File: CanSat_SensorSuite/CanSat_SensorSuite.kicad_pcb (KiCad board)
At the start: 4 copper layers, 100 x 80 mm, 42 parts, among them J13 Conn_02x03_Odd_Even, J2 USBC_Conn, J4 Pin_01x02, U1 RP2350_80QFN, U2 S25FL128, U3 NCP1117_3.3, X1 ABM8-272-T3

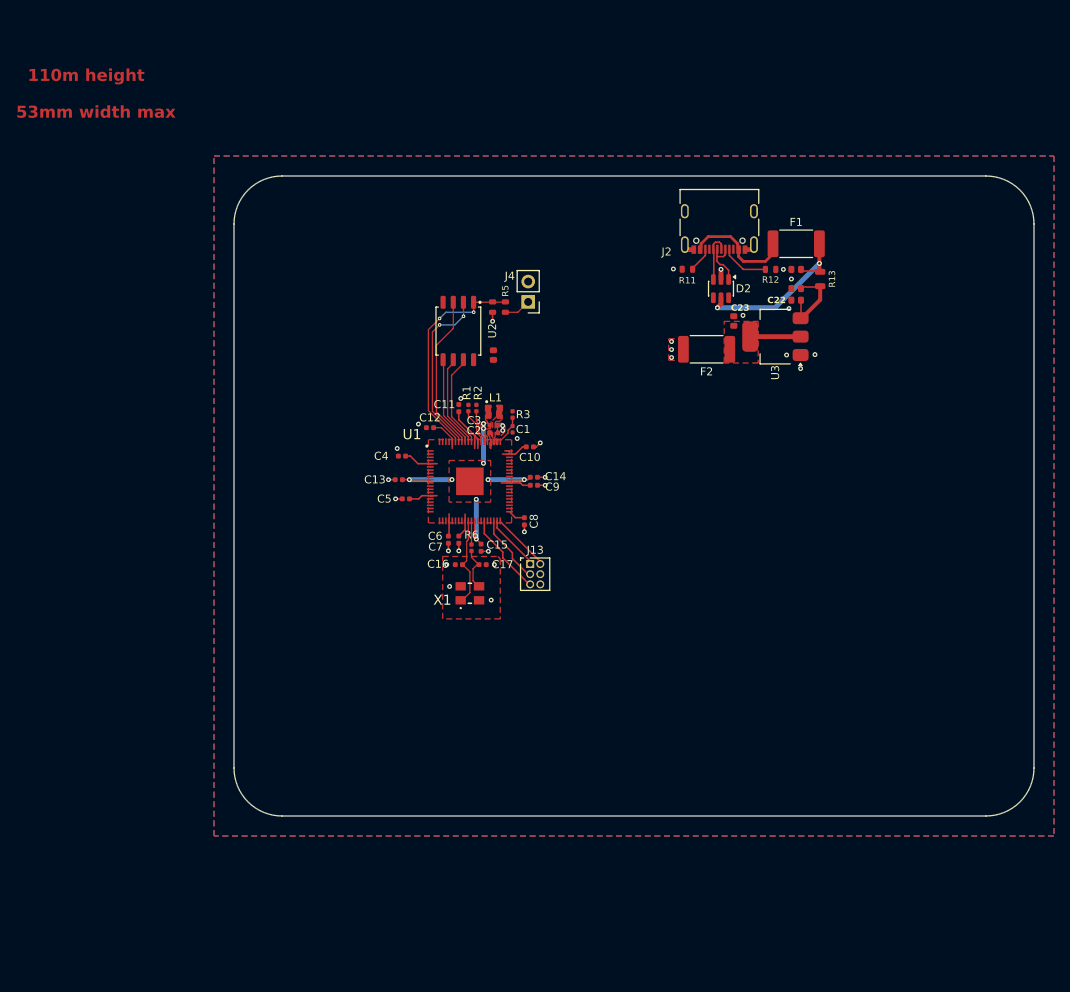
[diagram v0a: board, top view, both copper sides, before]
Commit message: Major sensor suite board changes, start of PCB layout
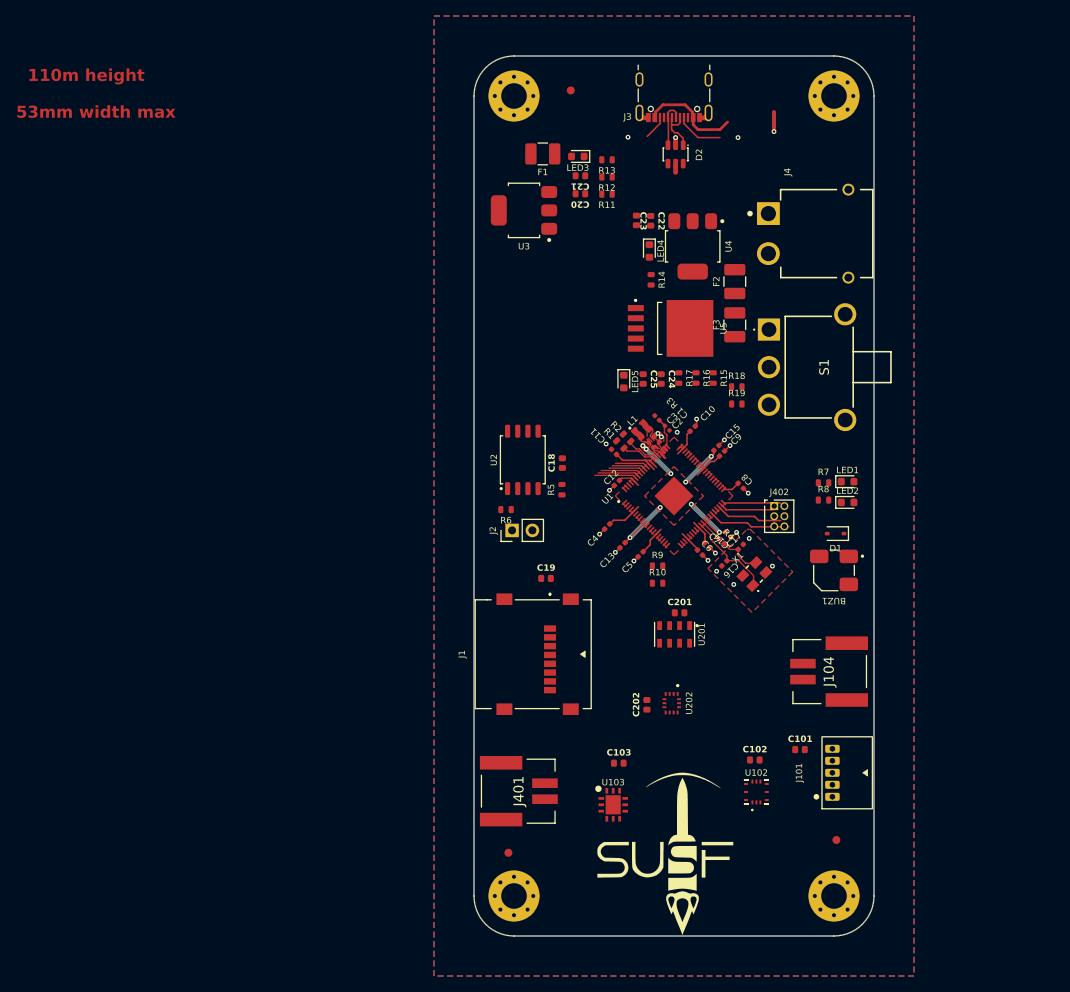
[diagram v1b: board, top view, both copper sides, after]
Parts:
- removed J13: Conn_02x03_Odd_Even, 0_Connectors:PinHeader_2x03_P1.27mm_Vertical
- added BUZ1: ~, 0_Passives:BUZZER,5x5mm, F.Cu at (175.0, 99.3)
- added C101: 100nF, 0_Capacitors:C_0603_1608_DensityHigh, F.Cu at (170.8, 121.7)
- added C102: 100nF, 0_Capacitors:C_0603_1608_DensityHigh, F.Cu at (165.1, 123.0)
- added C103: 100nF, 0_Capacitors:C_0603_1608_DensityHigh, F.Cu at (148.1, 123.4)
- added C19: 100nF, 0_Capacitors:C_0603_1608_DensityHigh, F.Cu at (139.0, 100.3)
- added C201: 100nF, 0_Capacitors:C_0603_1608_DensityHigh, F.Cu at (155.7, 104.6)
- added C202: 100nF, 0_Capacitors:C_0603_1608_DensityHigh, F.Cu at (151.6, 116.1)
- added C24: 10uF, 0_Capacitors:C_0603_1608_DensityHigh, F.Cu at (153.4, 75.4)
- added C25: 10uF, 0_Capacitors:C_0603_1608_DensityHigh, F.Cu at (151.2, 75.4)
- added D1: ~, 0_Passives:D_SOD-323, F.Cu at (175.2, 94.7)
- added F3: Fuse, 0_Power:Fuse_1210_3225Metric, F.Cu at (162.6, 68.6)
- added FID301: Fiducial Marker, 0_Mechanical:Fiducial_1mm_Mask2mm, F.Cu at (134.3, 134.6)
- added FID302: Fiducial Marker, 0_Mechanical:Fiducial_1mm_Mask2mm, F.Cu at (175.3, 133.0)
- added FID303: Fiducial Marker, 0_Mechanical:Fiducial_1mm_Mask2mm, F.Cu at (142.1, 39.3)
- added G***: LOGO, SUSF_Footprint_Lib:SUSF_LOGO_BIG, F.Cu at (154.4, 134.8)
- added J1: Micro_SD_Card, 0_Connectors:Molex_472192001_uSD, F.Cu at (137.7, 109.8)
- added J101: SPS30, 0_Connectors:JST-S5B-ZR, F.Cu at (174.8, 127.6)
- added J104: Molex_01x02, 0_Connectors:502352_0201, F.Cu at (173.9, 112.0)
- added J3: USBC_Conn, 0_Connectors:USB4105_GCT, F.Cu at (155.0, 39.3)
- added J401: Molex_01x02, 0_Connectors:502352_0201, F.Cu at (136.1, 126.9)
- added J402: Conn_02x03, 0_Connectors:PinHeader_2x03_P1.27mm_Vertical, F.Cu at (167.5, 91.3)
- added LED1: Green, 0_Passives:LED_0603_1608Metric, F.Cu at (176.7, 88.2)
- added LED2: Red, 0_Passives:LED_0603_1608Metric, F.Cu at (176.7, 90.8)
- added LED3: Red, 0_Passives:LED_0603_1608Metric, F.Cu at (143.0, 47.6)
- added LED4: Red, 0_Passives:LED_0603_1608Metric, F.Cu at (151.9, 59.4)
- added LED5: Red, 0_Passives:LED_0603_1608Metric, F.Cu at (148.7, 75.7)
- added MH301: M3_MountingHole_Pad, 0_Mechanical:MountingHole_3.2mm_M3_Pad_Via, F.Cu at (135.0, 140.0)
- added MH302: M3_MountingHole_Pad, 0_Mechanical:MountingHole_3.2mm_M3_Pad_Via, F.Cu at (175.0, 140.0)
- added MH303: M3_MountingHole_Pad, 0_Mechanical:MountingHole_3.2mm_M3_Pad_Via, F.Cu at (135.0, 40.0)
- added MH304: M3_MountingHole_Pad, 0_Mechanical:MountingHole_3.2mm_M3_Pad_Via, F.Cu at (175.0, 40.0)
- added R10: 4.7kR, 0_Resistors:R_0603_1608_DensityHigh, F.Cu at (152.9, 100.9)
- added R14: 51R, 0_Resistors:R_0603_1608_DensityHigh, F.Cu at (152.1, 63.0)
- added R15: ???R, 0_Resistors:R_0603_1608_DensityHigh, F.Cu at (159.9, 75.2)
- added R16: ???R, 0_Resistors:R_0603_1608_DensityHigh, F.Cu at (157.8, 75.2)
- added R17: 51R, 0_Resistors:R_0603_1608_DensityHigh, F.Cu at (155.6, 75.2)
- added R18: 470kR, 0_Resistors:R_0603_1608_DensityHigh, F.Cu at (162.8, 76.3)
- added R19: 390kR, 0_Resistors:R_0603_1608_DensityHigh, F.Cu at (162.8, 78.5)
- added R7: 51R, 0_Resistors:R_0603_1608_DensityHigh, F.Cu at (173.7, 88.4)
- added R8: 51R, 0_Resistors:R_0603_1608_DensityHigh, F.Cu at (173.7, 90.5)
- added R9: 4.7kR, 0_Resistors:R_0603_1608_DensityHigh, F.Cu at (152.9, 98.8)
- added S1: SPST_1101M2S3AQE2, 0_Power:1101M2S3AQE2, F.Cu at (166.9, 69.2)
- added U102: ZMOD4410AI1R, 0_Sensors:ZMOD4410AI1R, F.Cu at (165.3, 127.0)
- added U103: STC31-C-R3, 0_Sensors:STC31-C-R3, F.Cu at (147.4, 128.6)
- added U201: MS560702BA03-50, 0_Sensors:MS5607-02BA03, F.Cu at (155.1, 107.3)
- added U202: LSM6DSOQTR, 0_Sensors:LSM6DSOQTR, F.Cu at (154.7, 115.9)
- added U4: NCP1117_3.3, 0_Power:SOT-223-3_TabPin2, F.Cu at (157.3, 58.8)
- added U5: MIC29302AWD, 0_Power:MIC29302AWD, F.Cu at (157.0, 69.0)
- C20, C21: value DNP -> 10nF
- F1, F2: footprint 0_Passives:Fuse_2512_6332Metric -> 0_Power:Fuse_1210_3225Metric
- J2: value USBC_Conn -> Pin_01x02; footprint 0_Connectors:USB4105_GCT -> 0_Connectors:PinHeader_1x02_P2.54mm_Vertical
- J4: value Pin_01x02 -> XT30_THT_H; footprint 0_Connectors:PinHeader_1x02_P2.54mm_Vertical -> 0_Connectors:XT30_THT_H
- L1: value 1uH -> 3.3uH
- R1, R2, R6: footprint 0_Resistors:R_0402_1005_DensityHigh -> 0_Resistors:R_0603_1608_DensityHigh
- R13: value 0R -> 51R; footprint 0_Resistors:R_0805_2012_DensityHigh -> 0_Resistors:R_0603_1608_DensityHigh
- R4: value 10kR -> 1kR; footprint 0_Resistors:R_0603_1608_DensityHigh -> 0_Resistors:R_0402_1005_DensityMedium
- R5: value 1kR -> 10kR
- U1: value RP2350_80QFN -> RP2350B
- moved J2 46.5 mm to (134.8, 94.3), turned to 90 degrees
- moved R4 40.9 mm to (160.9, 95.7), turned to -45 degrees
- moved X1 35.6 mm to (165.0, 99.8), turned to 45 degrees
- moved U3 35.2 mm to (136.2, 54.3)
- moved F1 33.6 mm to (138.6, 47.2)
- moved C16 33.2 mm to (161.3, 98.4), turned to -135 degrees
- moved C17 32.3 mm to (163.3, 96.4), turned to 45 degrees
- moved J4 32.0 mm to (166.8, 54.7), turned to -90 degrees
- moved C15 32.0 mm to (160.3, 84.0), turned to -135 degrees
- moved C6 31.5 mm to (158.3, 97.1), turned to -45 degrees
- moved C7 31.1 mm to (159.2, 96.2), turned to -45 degrees
- moved R13 30.5 mm to (146.6, 48.0), turned to 180 degrees
- moved C21 30.4 mm to (143.3, 50.0), turned to 180 degrees
- moved C5 30.1 mm to (150.8, 97.3), turned to -135 degrees
- moved C13 29.1 mm to (148.6, 96.2), turned to 45 degrees
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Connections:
- net /CCT Board Schematic/MCU & Peripherals/QSPI_SCLK renamed /Sensor Board Schematic/MCU & Peripherals/QSPI_SCLK
- net /CCT Board Schematic/MCU & Peripherals/QSPI_SD0 renamed /Sensor Board Schematic/MCU & Peripherals/QSPI_SD0
- net /CCT Board Schematic/MCU & Peripherals/QSPI_SD1 renamed /Sensor Board Schematic/MCU & Peripherals/QSPI_SD1
- net /CCT Board Schematic/MCU & Peripherals/QSPI_SD2 renamed /Sensor Board Schematic/MCU & Peripherals/QSPI_SD2
- net /CCT Board Schematic/MCU & Peripherals/QSPI_SD3 renamed /Sensor Board Schematic/MCU & Peripherals/QSPI_SD3
- net /CCT Board Schematic/MCU & Peripherals/USB_DM renamed /Sensor Board Schematic/MCU & Peripherals/USB_DM
- net /CCT Board Schematic/MCU & Peripherals/USB_DP renamed /Sensor Board Schematic/MCU & Peripherals/USB_DP
- net /CCT Board Schematic/MCU & Peripherals/VREG_AVDD renamed /Sensor Board Schematic/MCU & Peripherals/VREG_AVDD
- net /CCT Board Schematic/MCU & Peripherals/VREG_LX renamed /Sensor Board Schematic/MCU & Peripherals/VREG_LX
- net /CCT Board Schematic/MCU & Peripherals/XIN renamed /Sensor Board Schematic/MCU & Peripherals/XIN
- C21 pad 1: GND -> +3V3
- C21 pad 2: VBUS_F -> GND
- C22 pad 2: VBUS_F -> VREG
- C23 pad 1: Net-(U3-VO) -> +3V3
- D2 pad 1: /CCT Board Schematic/USBC/D- -> /Sensor Board Schematic/USBC & Battery Supply/D-
- D2 pad 3: /CCT Board Schematic/USBC/D+ -> /Sensor Board Schematic/USBC & Battery Supply/D+
- D2 pad 4: /CCT Board Schematic/USBC/USB_D+ -> /Sensor Board Schematic/MCU & Peripherals/USB_D+
- D2 pad 6: /CCT Board Schematic/USBC/USB_D- -> /Sensor Board Schematic/MCU & Peripherals/USB_D-
- F1 pad 2: /CCT Board Schematic/USBC/VBUS_PF -> /Sensor Board Schematic/USBC & Battery Supply/VBUS_PF
- F2 pad 1: +3V3 -> /Sensor Board Schematic/USBC & Battery Supply/BAT_CONN_OUT
- F2 pad 2: Net-(U3-VO) -> VBUS
- J4 pad 1: /CCT Board Schematic/MCU & Peripherals/~{USB_BOOT} -> /Sensor Board Schematic/USBC & Battery Supply/BAT_CONN_IN
- R1 pad 1: /CCT Board Schematic/MCU & Peripherals/USB_D+ -> /Sensor Board Schematic/MCU & Peripherals/USB_D+
- R11 pad 2: /CCT Board Schematic/USBC/CC2 -> /Sensor Board Schematic/USBC & Battery Supply/CC2
- R12 pad 1: /CCT Board Schematic/USBC/CC1 -> /Sensor Board Schematic/USBC & Battery Supply/CC1
- R13 pad 1: VBUS -> GND
- R13 pad 2: VBUS_F -> Net-(LED3-K)
- R2 pad 1: /CCT Board Schematic/MCU & Peripherals/USB_D- -> /Sensor Board Schematic/MCU & Peripherals/USB_D-
- R4 pad 1: /CCT Board Schematic/MCU & Peripherals/QSPI_CS -> /Sensor Board Schematic/MCU & Peripherals/XOUT
- R4 pad 2: +3V3 -> Net-(C17-Pad1)
- R5 pad 1: /CCT Board Schematic/MCU & Peripherals/QSPI_CS -> /Sensor Board Schematic/MCU & Peripherals/QSPI_CS
- R5 pad 2: /CCT Board Schematic/MCU & Peripherals/~{USB_BOOT} -> +3V3
- R6 pad 1: /CCT Board Schematic/MCU & Peripherals/XOUT -> /Sensor Board Schematic/MCU & Peripherals/QSPI_CS
- R6 pad 2: Net-(C17-Pad1) -> /Sensor Board Schematic/MCU & Peripherals/~{USB_BOOT}
- U1 pad 1: /CCT Board Schematic/MCU & Peripherals/FIRE_SIGNAL -> /Sensor Board Schematic/MCU & Peripherals/SD_DAT1
- U1 pad 11: /CCT Board Schematic/MCU & Peripherals/Servo2_PWM -> unconnected-(U1A-GPIO12-Pad11)
- U1 pad 12: /CCT Board Schematic/MCU & Peripherals/SD_DAT1 -> unconnected-(U1A-GPIO13-Pad12)
- U1 pad 13: /CCT Board Schematic/MCU & Peripherals/Servo3_PWM -> unconnected-(U1A-GPIO14-Pad13)
- U1 pad 14: /CCT Board Schematic/MCU & Peripherals/SD_DAT0 -> unconnected-(U1A-GPIO15-Pad14)
- U1 pad 16: /CCT Board Schematic/MCU & Peripherals/SD_CLK -> unconnected-(U1A-GPIO16-Pad16)
- U1 pad 17: /CCT Board Schematic/MCU & Peripherals/SD_CMD -> unconnected-(U1A-GPIO17-Pad17)
- U1 pad 18: /CCT Board Schematic/MCU & Peripherals/SD_DAT3 -> unconnected-(U1A-GPIO18-Pad18)
- U1 pad 19: /CCT Board Schematic/MCU & Peripherals/SD_DAT2 -> unconnected-(U1A-GPIO19-Pad19)
- U1 pad 2: /CCT Board Schematic/MCU & Peripherals/ARM_SIGNAL -> /Sensor Board Schematic/MCU & Peripherals/SD_DAT0
- U1 pad 20: /CCT Board Schematic/MCU & Peripherals/I2C_SDA -> /Sensor Board Schematic/AtmoSensors/I2C_SDA
- U1 pad 21: /CCT Board Schematic/MCU & Peripherals/I2C_SCL -> /Sensor Board Schematic/AtmoSensors/I2C_SCL
- U1 pad 3: /CCT Board Schematic/MCU & Peripherals/FILL_SIGNAL -> /Sensor Board Schematic/MCU & Peripherals/SD_CLK
- U1 pad 31: /CCT Board Schematic/MCU & Peripherals/XOUT -> /Sensor Board Schematic/MCU & Peripherals/XOUT
- U1 pad 35: /CCT Board Schematic/MCU & Peripherals/RUN -> /Sensor Board Schematic/MCU & Peripherals/RUN
- U1 pad 38: /CCT Board Schematic/MCU & Peripherals/GPIO30 -> /Sensor Board Schematic/MCU & Peripherals/GPIO30
- U1 pad 39: /CCT Board Schematic/MCU & Peripherals/GPIO31 -> /Sensor Board Schematic/MCU & Peripherals/GPIO31
- U1 pad 4: /CCT Board Schematic/MCU & Peripherals/RJ45_LED2 -> /Sensor Board Schematic/MCU & Peripherals/SD_CMD
- U1 pad 40: /CCT Board Schematic/MCU & Peripherals/GPIO32 -> /Sensor Board Schematic/MCU & Peripherals/GPIO32
- U1 pad 44: /CCT Board Schematic/MCU & Peripherals/STATUS_BUZZER- -> /Sensor Board Schematic/MCU & Peripherals/STATUS_BUZZER-
- U1 pad 45: /CCT Board Schematic/MCU & Peripherals/STATUS_BUZZER+ -> /Sensor Board Schematic/MCU & Peripherals/STATUS_BUZZER+
- U1 pad 47: /CCT Board Schematic/MCU & Peripherals/STATUS_LED_R -> /Sensor Board Schematic/MCU & Peripherals/STATUS_LED_R
- U1 pad 48: /CCT Board Schematic/MCU & Peripherals/STATUS_LED_G -> /Sensor Board Schematic/MCU & Peripherals/STATUS_LED_G
- U1 pad 54: /CCT Board Schematic/MCU & Peripherals/PYRO_SENSE -> unconnected-(U1A-GPIO43_ADC3-Pad54)
- U1 pad 55: /CCT Board Schematic/MCU & Peripherals/PYRO_IN -> unconnected-(U1A-GPIO44_ADC4-Pad55)
- U1 pad 56: /CCT Board Schematic/MCU & Peripherals/PYRO_SEN -> unconnected-(U1A-GPIO45_ADC5-Pad56)
- U1 pad 58: /CCT Board Schematic/VBAT_sense -> /Sensor Board Schematic/MCU & Peripherals/VBAT_sense
- U1 pad 6: /CCT Board Schematic/MCU & Peripherals/RS485_TX -> /Sensor Board Schematic/MCU & Peripherals/SD_DAT3
- U1 pad 7: /CCT Board Schematic/MCU & Peripherals/RS485_RX -> /Sensor Board Schematic/MCU & Peripherals/SD_DAT2
- U1 pad 75: /CCT Board Schematic/MCU & Peripherals/QSPI_CS -> /Sensor Board Schematic/MCU & Peripherals/QSPI_CS
- U1 pad 8: /CCT Board Schematic/MCU & Peripherals/RJ45_LED1 -> unconnected-(U1A-GPIO10-Pad8)
- U1 pad 9: /CCT Board Schematic/MCU & Peripherals/Servo1_PWM -> unconnected-(U1A-GPIO11-Pad9)
- U2 pad 1: /CCT Board Schematic/MCU & Peripherals/QSPI_CS -> /Sensor Board Schematic/MCU & Peripherals/QSPI_CS
- U3 pad 2: Net-(U3-VO) -> +3V3
- U3 pad 3: VBUS_F -> VBUS
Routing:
- net /CCT Board Schematic/MCU & Peripherals/QSPI_CS: track 27.2 -> 0.00 mm, vias 2 -> 0
- net VBUS: track 21.9 -> 3.26 mm, vias 2 -> 1
- net /Sensor Board Schematic/MCU & Peripherals/QSPI_SD1: track 21.5 -> 5.17 mm, vias 2 -> 0
- net /Sensor Board Schematic/MCU & Peripherals/QSPI_SD2: track 19.6 -> 5.06 mm
- net /Sensor Board Schematic/USBC & Battery Supply/VBUS_PF: track 0.00 -> 12.2 mm
- net /CCT Board Schematic/USBC/VBUS_PF: track 12.2 -> 0.00 mm
- net /Sensor Board Schematic/MCU & Peripherals/RUN: track 0.00 -> 10.3 mm
- net /CCT Board Schematic/MCU & Peripherals/RUN: track 10.3 -> 0.00 mm
- net VBUS_F: track 8.85 -> 0.00 mm
- net /CCT Board Schematic/MCU & Peripherals/GPIO30: track 8.43 -> 0.00 mm
- net /Sensor Board Schematic/MCU & Peripherals/GPIO30: track 0.00 -> 8.43 mm
- net /Sensor Board Schematic/MCU & Peripherals/QSPI_SD3: track 11.4 -> 4.14 mm
- net /Sensor Board Schematic/MCU & Peripherals/GPIO32: track 0.00 -> 7.08 mm
- net /CCT Board Schematic/MCU & Peripherals/GPIO32: track 7.08 -> 0.00 mm
- net /Sensor Board Schematic/MCU & Peripherals/QSPI_SD0: track 11.3 -> 4.37 mm
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- added copper zone on F.Cu, net (none)
- removed copper zone on F.Cu, net /Sensor Board Schematic/MCU & Peripherals/VREG_LX
- removed copper zone on F.Cu, net Net-(U3-VO)
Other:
- board size 100 x 80 mm -> 50 x 110 mm
- board text removed: "??? ??? ???"
- board text removed: "??? ??? ??? ??? ??? (slot) ??? ??? ??? ??? ???"
- board text removed: "???mm ???mm ???mm ???mm ???mm ???mm ???mm ???mm ???mm ???mm"
- board text removed: "ASSEMBLY NOTES (UNLESS OTHERWISE SPECIFIED) 1) DO NOT POPULATE PARTS ARE MARKED WITH A RED CROSS. 2) DO NOT POPULATE PARTS ARE NOT PRESENT IN THE BOM. 3) IF CONFLICTING INFORMATION IS FOUND BETWEEN THE ASSEMBLY FILE AND BOM, BOM SHOULD BE USED AS THE MAIN SOURCE."
- board text removed: "Back Side"
- board text removed: "Bottom Assembly (Scale 1:1)"
- board text removed: "Bottom Test Points (Scale 1:1)"
- board text removed: "Bottom View"
- board text removed: "Components"
- board text removed: "Count"
- board text removed: "Drill Drawing (Top View) (Scale 1:1)"
- board text removed: "Front Side"
- board text removed: "Hole Size"
- board text removed: "Net"
- board text removed: "Plated"
- board text removed: "Plated Plated Plated Plated Plated Plated Plated Plated Plated Unplated"
- board text removed: "Ref."
- board text removed: "Symbol"
- board text removed: "THT SMD Total"
- board text removed: "TP? TP? TP?"
- board text removed: "Top Assembly (Scale 1:1)"
- board text removed: "Top Test Points (Scale 1:1)"
- board text removed: "Top View"
- board text removed: "Total"
- board text removed: "Type"
- board text removed: "X"
- board text removed: "X [mm]"
- board text removed: "Y"
- board text removed: "Y [mm]"
